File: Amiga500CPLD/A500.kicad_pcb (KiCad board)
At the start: 2 copper layers, 64.5 x 111 mm, 13 parts, among them J1 Raspberry_Pi_2_3, J2 Conn_01x01, U1 DeniseSocket, U2 DenisePins, U3 XC9572VQ44

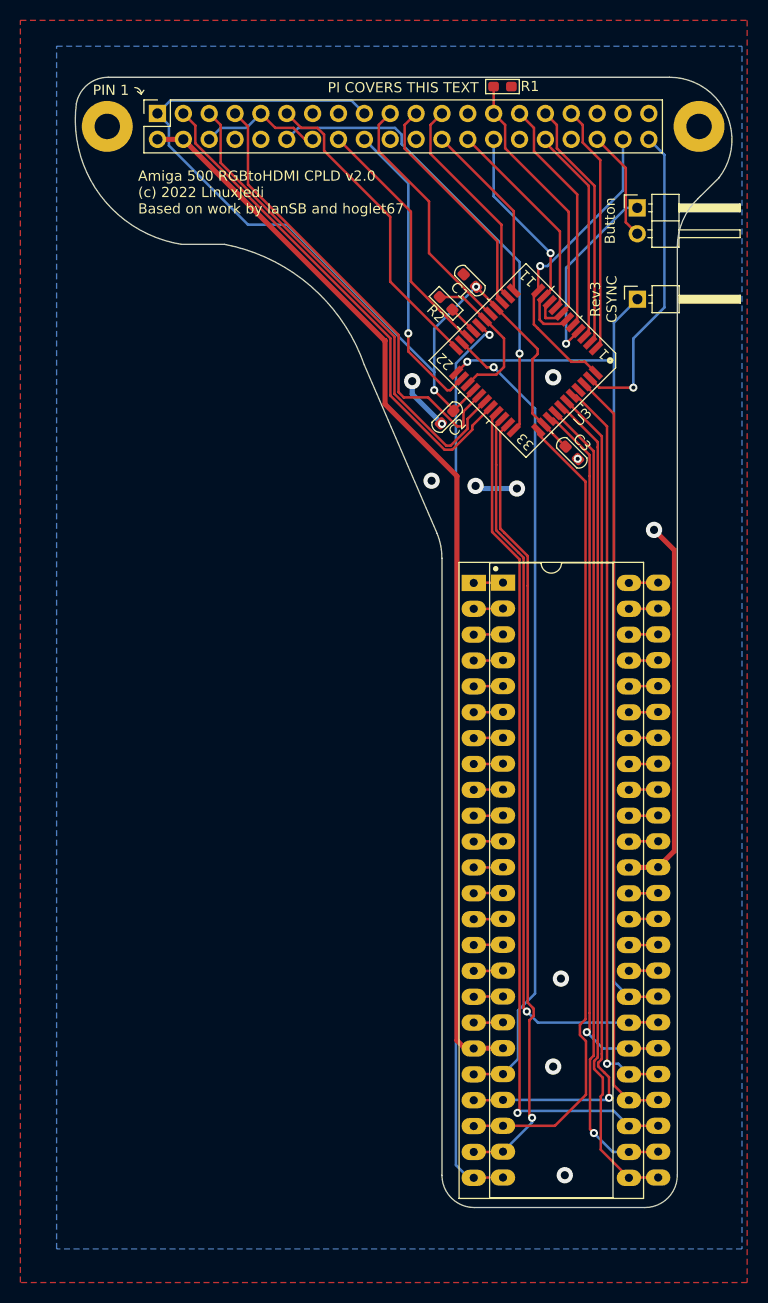
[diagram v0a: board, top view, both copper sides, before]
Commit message: Update design to include audio
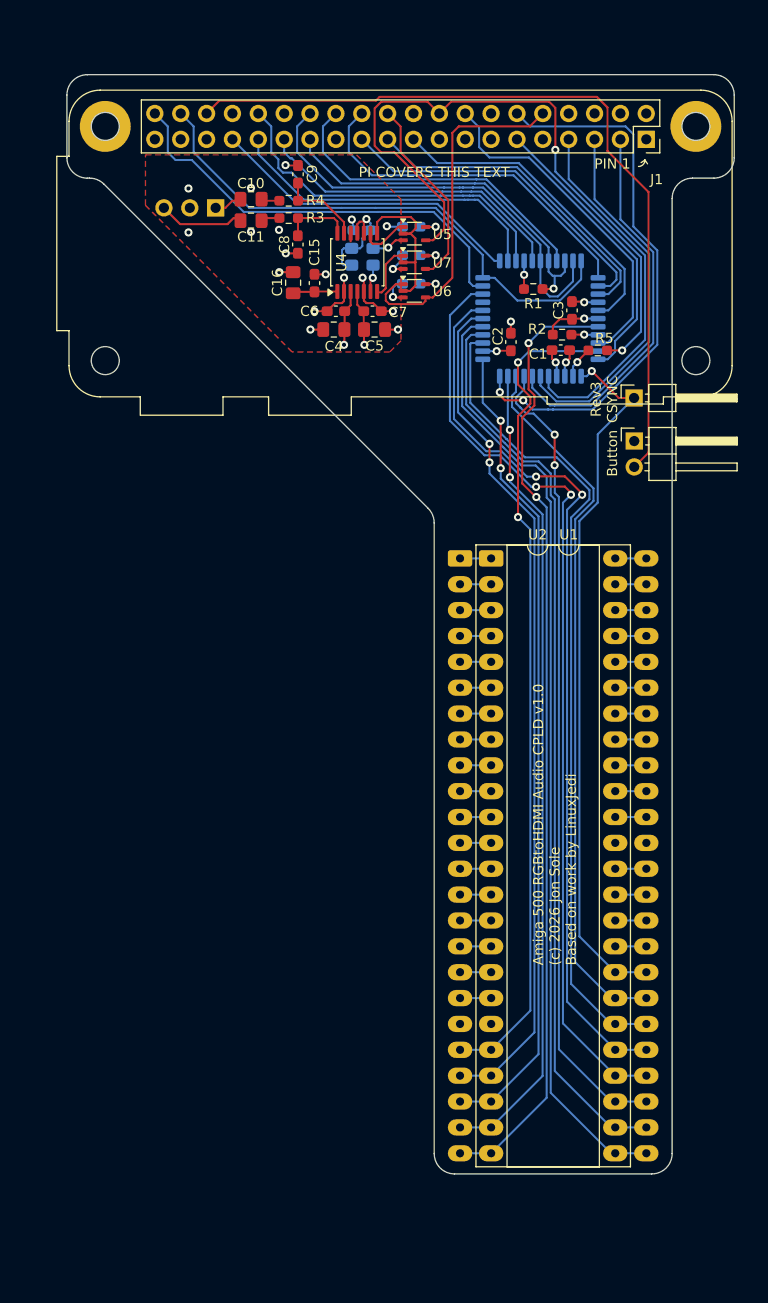
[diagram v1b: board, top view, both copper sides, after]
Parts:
- added C10: 2.2uF, Capacitor_SMD:C_0805_2012Metric_Pad1.18x1.45mm_HandSolder, F.Cu at (68.9, 31.3)
- added C11: 2.2uF, Capacitor_SMD:C_0805_2012Metric_Pad1.18x1.45mm_HandSolder, F.Cu at (68.9, 33.4)
- added C12: 0.1uF, Capacitor_SMD:C_0603_1608Metric_Pad1.08x0.95mm_HandSolder, B.Cu at (84.6, 34.0)
- added C13: 0.1uF, Capacitor_SMD:C_0603_1608Metric_Pad1.08x0.95mm_HandSolder, B.Cu at (84.6, 36.8)
- added C14: 0.1uF, Capacitor_SMD:C_0603_1608Metric_Pad1.08x0.95mm_HandSolder, B.Cu at (84.6, 39.6)
- added C15: 0.1uF, Capacitor_SMD:C_0603_1608Metric_Pad1.08x0.95mm_HandSolder, F.Cu at (75.1, 39.5)
- added C16: 10uF, Capacitor_SMD:C_0805_2012Metric_Pad1.18x1.45mm_HandSolder, F.Cu at (73.0, 39.5)
- added C17: 0.01uF, Capacitor_SMD:C_0603_1608Metric_Pad1.08x0.95mm_HandSolder, B.Cu at (79.8, 34.3)
- added C4: 10uF, Capacitor_SMD:C_0805_2012Metric_Pad1.18x1.45mm_HandSolder, F.Cu at (77.0, 44.1)
- added C5: 10uF, Capacitor_SMD:C_0805_2012Metric_Pad1.18x1.45mm_HandSolder, F.Cu at (81.0, 44.1)
- added C6: 0.1uF, Capacitor_SMD:C_0603_1608Metric_Pad1.08x0.95mm_HandSolder, F.Cu at (77.2, 42.3)
- added C7: 0.1uF, Capacitor_SMD:C_0603_1608Metric_Pad1.08x0.95mm_HandSolder, F.Cu at (80.8, 42.3)
- added C8: 0.1uF, Capacitor_SMD:C_0603_1608Metric_Pad1.08x0.95mm_HandSolder, F.Cu at (73.5, 35.7)
- added C9: 0.1uF, Capacitor_SMD:C_0603_1608Metric_Pad1.08x0.95mm_HandSolder, F.Cu at (73.5, 28.8)
- added J3: Conn_01x03, Connector_PinHeader_2.54mm:PinHeader_1x03_P2.54mm_Horizontal, B.Cu at (65.4, 32.1)
- added R3: 470R, Resistor_SMD:R_0603_1608Metric_Pad0.98x0.95mm_HandSolder, F.Cu at (72.6, 33.1)
- added R4: 470R, Resistor_SMD:R_0603_1608Metric_Pad0.98x0.95mm_HandSolder, F.Cu at (72.6, 31.4)
- added R5: 550R, Resistor_SMD:R_0603_1608Metric_Pad0.98x0.95mm_HandSolder, F.Cu at (102.9, 46.1)
- added U4: PCM1808, Package_SO:TSSOP-14_4.4x5mm_P0.65mm, F.Cu at (79.3, 37.5)
- added U5: SN74LVC1G80, Package_TO_SOT_SMD:Texas_R-PDSO-G5_DCK-5, F.Cu at (84.9, 34.7)
- added U6: SN74LVC1G80, Package_TO_SOT_SMD:Texas_R-PDSO-G5_DCK-5, F.Cu at (84.9, 40.3)
- added U7: SN74LVC1G80, Package_TO_SOT_SMD:Texas_R-PDSO-G5_DCK-5, F.Cu at (84.9, 37.5)
- added Y2: ASE-xxxMHz, Oscillator:Oscillator_SMD_Abracon_ASE-4Pin_3.2x2.5mm, B.Cu at (79.8, 36.9)
- C1, C2, C3: footprint Capacitor_SMD_AKL:C_0603_1608Metric_Pad1.08x0.95mm -> Capacitor_SMD:C_0603_1608Metric_Pad1.08x0.95mm_HandSolder
- J1: footprint Connector_PinSocket_2.54mm:PinSocket_2x20_P2.54mm_Vertical -> Module:Raspberry_Pi_Zero_Socketed_THT_FaceDown_MountingHoles
- R1, R2: footprint Resistor_SMD_AKL:R_0603_1608Metric_Pad1.05x0.95mm -> Resistor_SMD:R_0603_1608Metric_Pad0.98x0.95mm_HandSolder
- U1: footprint Package_DIP_AKL:DIP-48_W15.24mm_Socket_LongPads -> Package_DIP:DIP-48_W15.24mm_LongPads
- U2: footprint Package_DIP_AKL:DIP-48_W15.24mm_LongPads -> Package_DIP:DIP-48_W15.24mm_LongPads
- U3: footprint Package_QFP_AKL:TQFP-44_10x10mm_P0.8mm -> Package_QFP:TQFP-44_10x10mm_P0.8mm; moved to B.Cu
- moved J1 48.1 mm to (107.7, 25.4), turned to -90 degrees
- moved JP1 22.9 mm to (106.5, 55.0)
- moved R1 20.1 mm to (96.6, 40.1), turned to 180 degrees
- moved C3 14.0 mm to (100.4, 42.2), turned to -90 degrees
- moved R2 11.8 mm to (99.4, 44.6), turned to 0 degrees
- moved C1 11.2 mm to (99.3, 46.1), turned to 0 degrees
- moved J2 9.71 mm to (106.5, 50.8)
- moved C2 9.68 mm to (94.4, 45.3), turned to 90 degrees
- moved U2 4.84 mm to (89.4, 66.6)
- moved U3 4.35 mm to (97.3, 43.0), turned to -90 degrees
- moved U1 2.96 mm to (92.5, 66.6)
- moved H1 0.31 mm to (112.6, 24.1)
- moved H2 0.20 mm to (54.6, 24.1)
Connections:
- net /CLKEN renamed /GPIO1_SPCLKEN
- net /GPIO0 renamed /GPIO0_SPDATA
- net /GPIO10 renamed /GPIO10_QUAD8
- net /GPIO11 renamed /GPIO11_QUAD9
- net /GPIO12 renamed /GPIO12_QUAD10
- net /GPIO13 renamed /GPIO13_QUAD11
- net /GPIO17 renamed /GPIO17_PSYNC
- net /GPIO18 renamed /GPIO18_VERSION
- net /GPIO2 renamed /GPIO2_QUAD0
- net /GPIO20 renamed /GPIO20_SPCLK
- net /GPIO21 renamed /GPIO21_CLK
- net /GPIO23 renamed /GPIO23_CSYNC
- net /GPIO3 renamed /GPIO3_QUAD1
- net /GPIO4 renamed /GPIO4_QUAD2
- net /GPIO5 renamed /GPIO5_QUAD3
- net /GPIO6 renamed /GPIO6_QUAD4
- net /GPIO7 renamed /GPIO7_QUAD5
- net /GPIO8 renamed /GPIO8_QUAD6
- net /GPIO9 renamed /GPIO9_QUAD7
- net /HSYNC renamed /CSYNC
- J1 pad 10: /GPIO15 -> /GPIO15_AUDCLK
- J1 pad 18: /GPIO24 -> /GPIO24_AUDDAT
- J1 pad 22: /GPIO25 -> /GPIO25_AUDLR
- R2 pad 1: /DETECT -> GND
- R2 pad 2: GND -> /DETECT
- U3 pad 24: /GPIO24 -> Net-(U3-TDO)
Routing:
- net VCC: track 107.1 -> 11.1 mm, vias 0 -> 1
- net /GPIO16: track 10.9 -> 78.0 mm
- net /GPIO24_AUDDAT: track 0.00 -> 66.5 mm, vias 0 -> 2
- net +3V3: track 97.6 -> 31.8 mm, vias 2 -> 8
- net GND: track 93.0 -> 49.3 mm, vias 12 -> 24
- net /GPIO15_AUDCLK: track 0.00 -> 34.6 mm
- net /GPIO24: track 29.9 -> 0.00 mm, vias 1 -> 0
- net /GPIO20_SPCLK: track 30.3 -> 52.4 mm, vias 1 -> 0
- net /CSYNC: track 89.0 -> 69.6 mm
- net /GPIO25_AUDLR: track 0.00 -> 19.1 mm
- net /GPIO1_SPCLKEN: track 23.5 -> 42.4 mm, vias 1 -> 0
- net /GPIO8_QUAD6: track 17.8 -> 35.0 mm
- net /G0: track 75.0 -> 92.0 mm, vias 0 -> 2
- net Net-(U4-BCK): track 0.00 -> 16.0 mm
- net /G1: track 72.7 -> 88.4 mm, vias 1 -> 2
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- added copper zone on In2.Cu, net +3V3
- added copper zone on In1.Cu, net GND
- added copper zone on In2.Cu, net VCC
- removed copper zone on B.Cu, net GND
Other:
- board size 64.5 x 111 mm -> 65.5 x 108 mm
- copper layers 2 -> 4
- board text added: "Amiga 500 RGBtoHDMI Audio CPLD v1.0 (c) 2026 Jon Sole Based on work by LinuxJedi"
- board text added: "L"
- board text added: "R"
- board text removed: "Amiga 500 RGBtoHDMI CPLD v2.0 (c) 2022 LinuxJedi Based on work by IanSB and hoglet67"
